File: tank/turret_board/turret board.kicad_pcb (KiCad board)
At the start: 2 copper layers, 50.6 x 28.8 mm, 26 parts, among them Q1 2N3904, Q2 2N3904, U1 KA378R33, U2 pixart_ir, Y1 Crystal_4pin

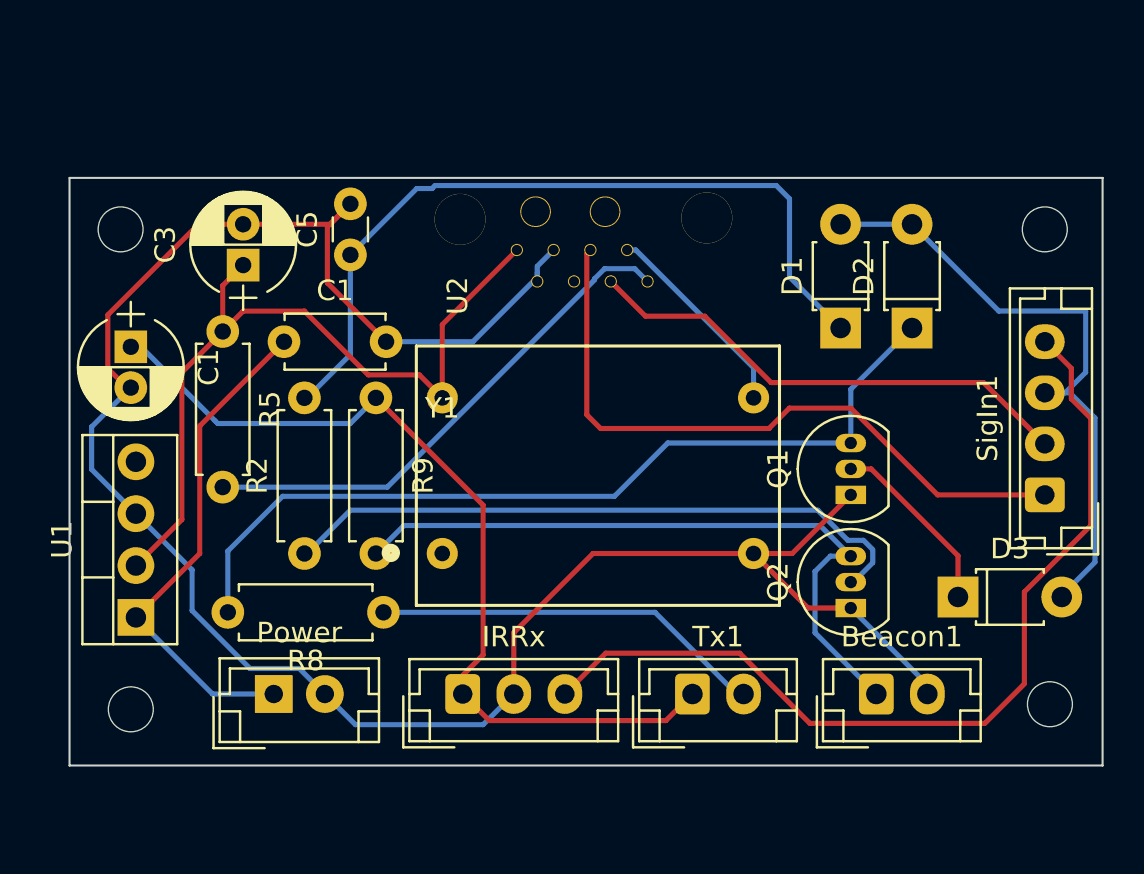
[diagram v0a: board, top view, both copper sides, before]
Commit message: and all that jazz
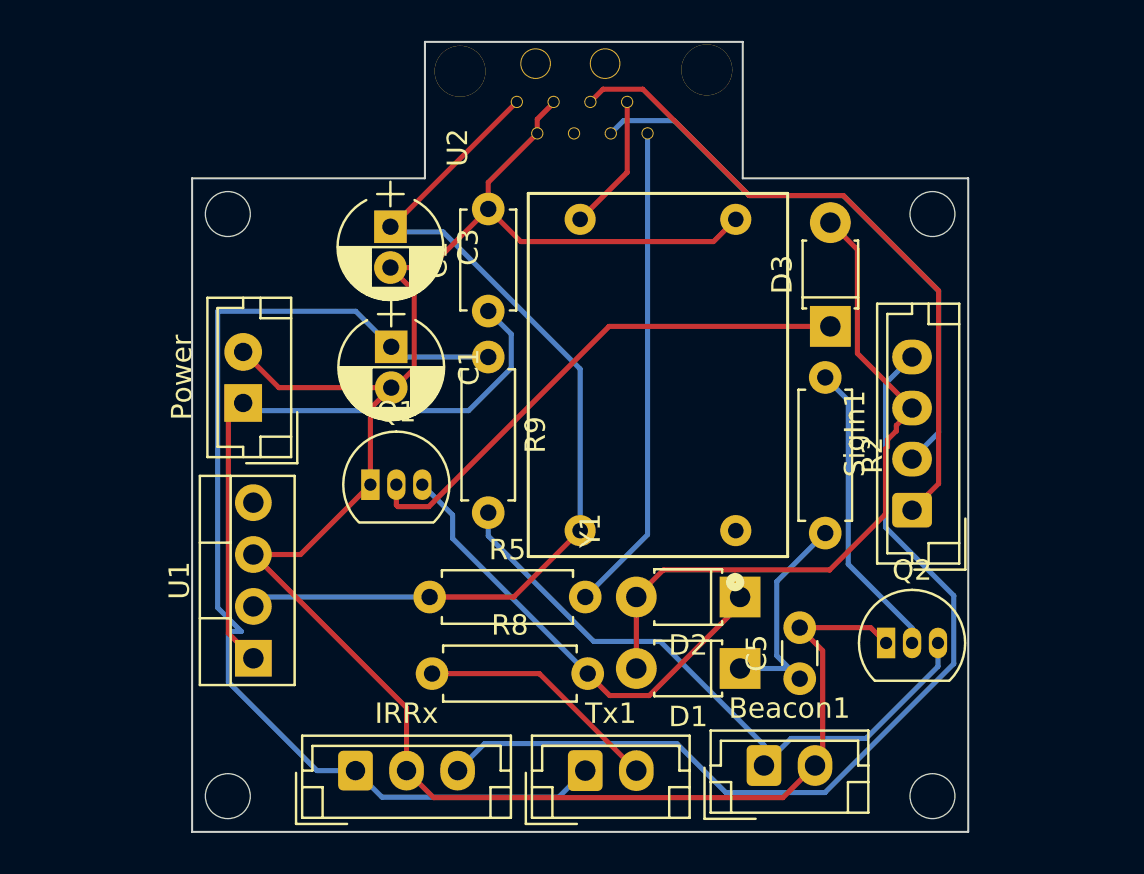
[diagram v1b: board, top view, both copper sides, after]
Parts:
- moved C5 30.2 mm to (212.5, 118.5)
- moved R2 26.9 mm to (213.8, 103.8), turned to 270 degrees
- moved Q1 23.5 mm to (191.5, 109.0), turned to 0 degrees
- moved D1 17.4 mm to (209.6, 118.0), turned to 180 degrees
- moved R5 16.5 mm to (194.4, 114.5), turned to 0 degrees
- moved D2 15.6 mm to (209.6, 114.5), turned to 180 degrees
- moved D3 14.7 mm to (214.0, 101.2), turned to 90 degrees
- moved Power 14.3 mm to (185.2, 105.0), turned to 90 degrees
- moved C1 12.8 mm to (192.5, 102.2)
- moved C1 10.1 mm to (197.2, 100.5), turned to 90 degrees
- moved Y1 9.37 mm to (201.8, 111.2), turned to 90 degrees
- moved C3 7.45 mm to (192.5, 96.4), turned to 270 degrees
- moved REF** 7.30 mm to (219.0, 124.2)
- moved U2 7.25 mm to (195.2, 92.5)
- moved SigIn1 6.54 mm to (218.0, 110.2)
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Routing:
- net Net-(C5-Pad1): track 38.6 -> 11.7 mm
- net Net-(D2-Pad1): track 42.6 -> 22.7 mm
- net Net-(D3-Pad1): track 9.03 -> 25.9 mm
- net Net-(Q2-Pad2): track 31.7 -> 14.8 mm
- net 5V: track 43.1 -> 53.7 mm
- net 3.3V: track 38.6 -> 46.3 mm
- net IRTx: track 19.3 -> 12.0 mm
- net Net-(C1-Pad1): track 24.8 -> 31.4 mm
- net SDA: track 24.5 -> 28.5 mm
- net GND: track 103.7 -> 99.8 mm
- net Net-(U2-Pad7): track 10.1 -> 6.70 mm
- net IRSig: track 31.6 -> 33.8 mm
- net Beacon: track 33.7 -> 31.6 mm
- net RESET: track 25.5 -> 24.0 mm
- net IRRx: track 44.6 -> 45.4 mm
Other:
- board size 50.6 x 28.8 mm -> 38 x 38.7 mm
- board text added: "Turret Board v0.7 Laser Tag Robot Tank M.I.A.R. Labs nick.groesz@gmail.com"
- board text removed: "Turret Board v0.6 Laser Tag Robot Tank M.I.A.R. Labs nick.groesz@gmail.com"
